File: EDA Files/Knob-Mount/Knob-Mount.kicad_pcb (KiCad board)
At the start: 2 copper layers, 184 x 42 mm, 3 parts, among them J1 Top Row, J2 Top Row

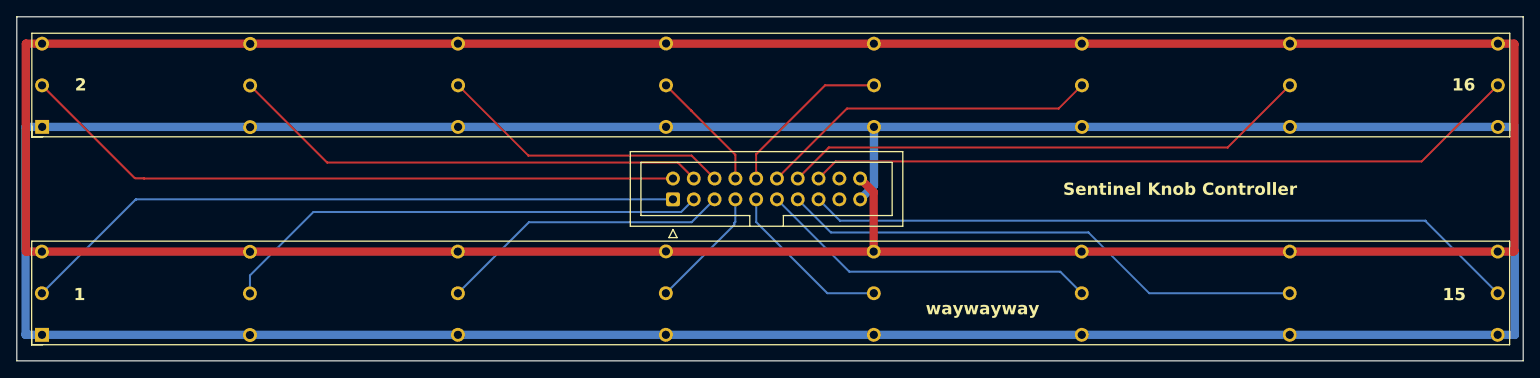
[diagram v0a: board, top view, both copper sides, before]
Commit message: Updates
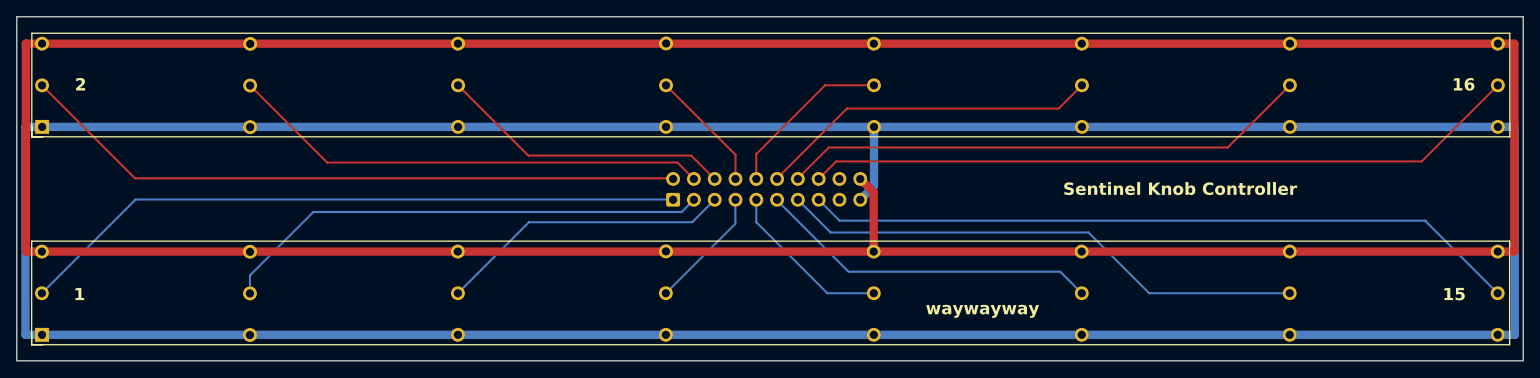
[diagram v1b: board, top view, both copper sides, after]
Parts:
- IDC1: moved to B.Cu
- moved IDC1 2.49 mm to (128.6, 84.8), turned to -90 degrees
